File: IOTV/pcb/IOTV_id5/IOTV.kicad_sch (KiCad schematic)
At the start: 24 parts, among them J1 Screw_Terminal_01x02, J2 Screw_Terminal_01x02, J3 Conn_01x04, J4 Conn_01x04, J5 Conn_01x04, J6 Conn_01x05, J7 JTAG, J8 UART, SW1 RST, SW2 Boot, U1 ESP32-WROOM-E, U2 G7DA-28 (Z)D3 8A/240V (3-32V)

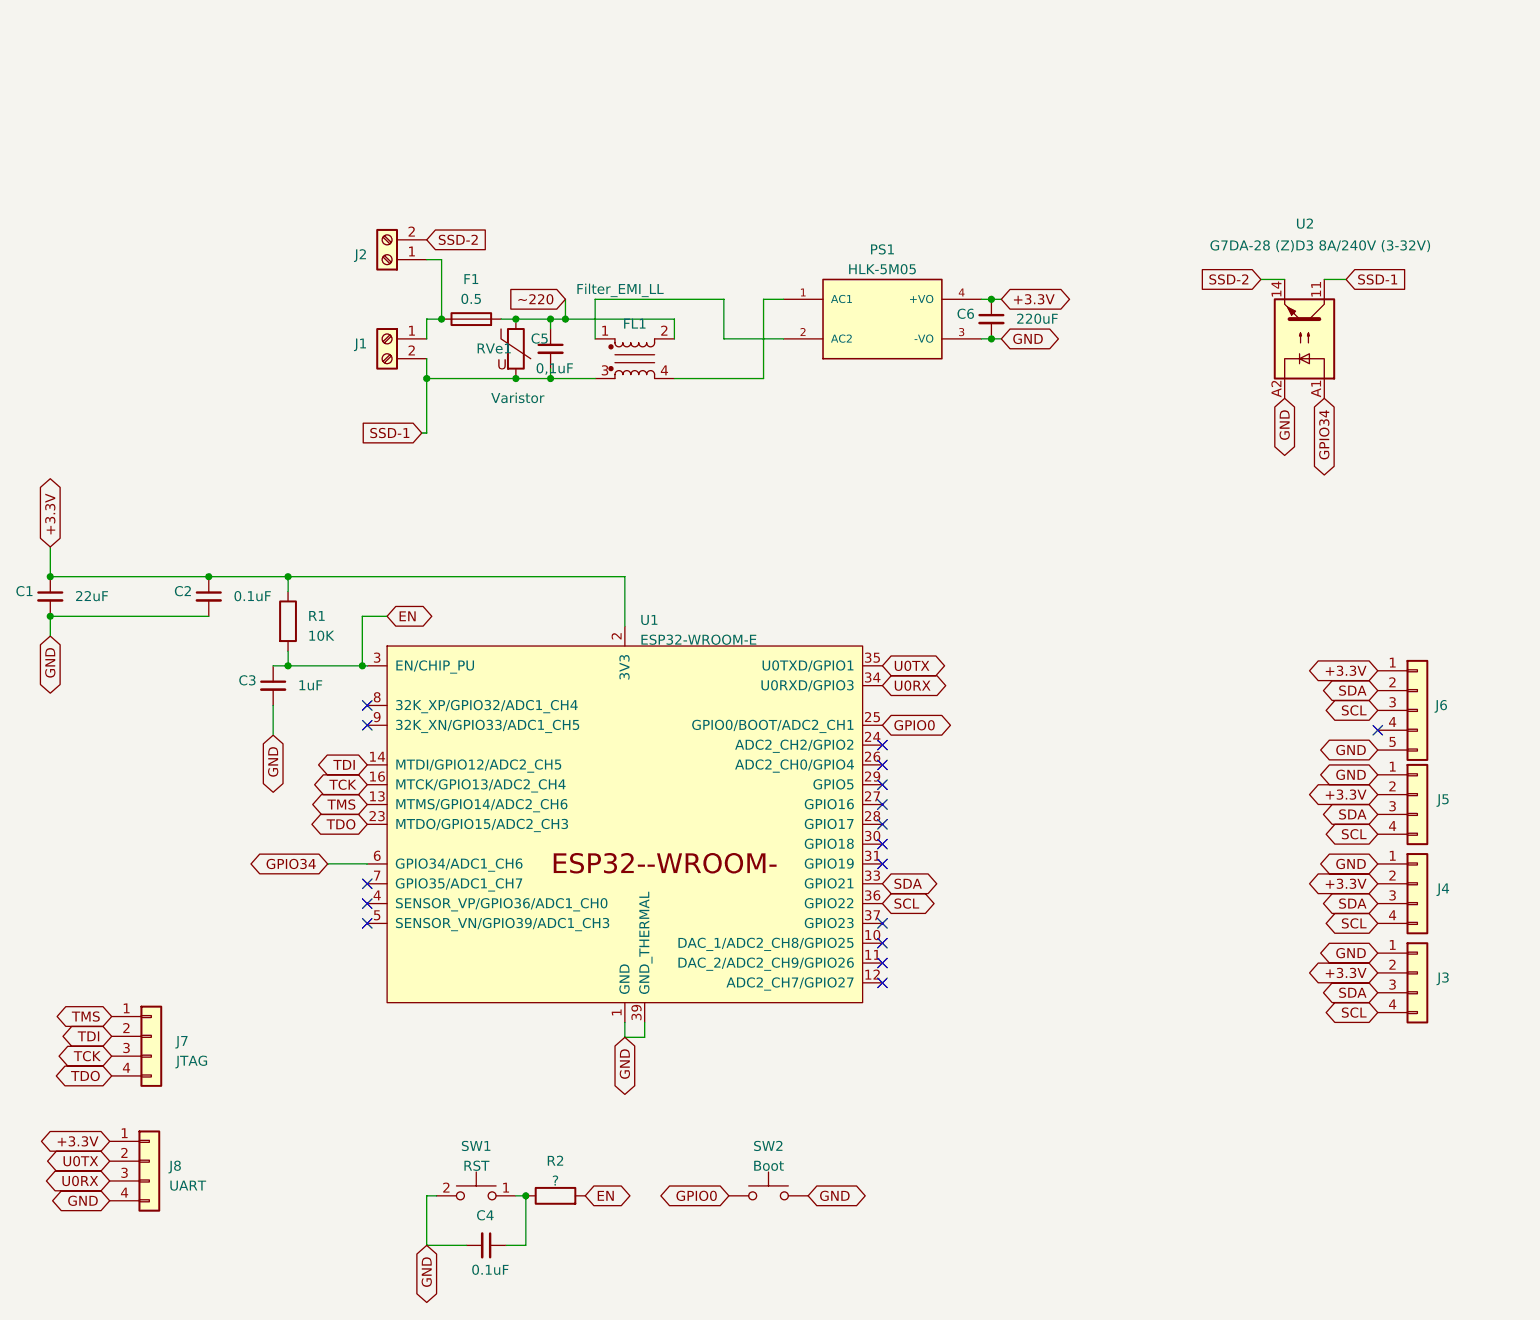
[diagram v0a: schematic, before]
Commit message: pcb id5 rev1.2
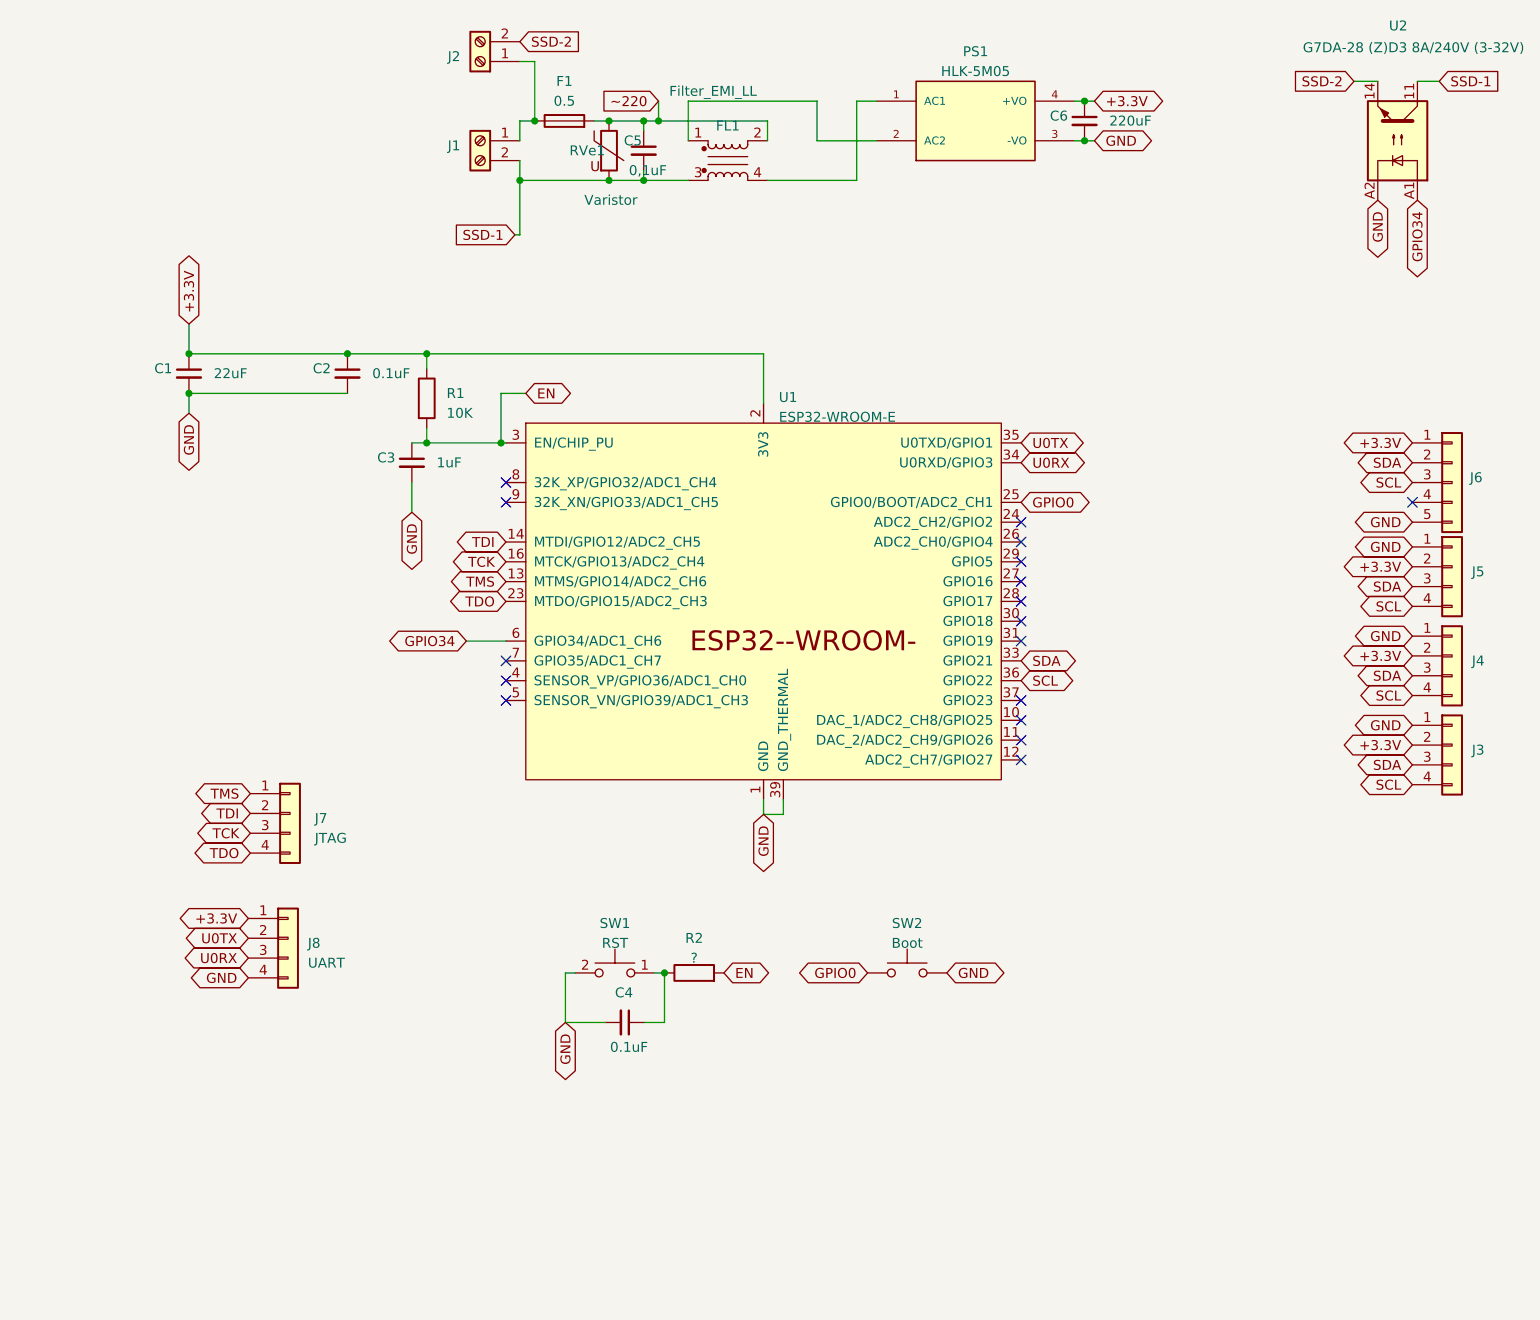
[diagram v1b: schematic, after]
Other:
- moved on the sheet: C1, C2, C3, C4, C5, C6, F1, FL1, J1, J2, J3, J4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
